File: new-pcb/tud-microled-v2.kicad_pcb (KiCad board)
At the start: 2 copper layers, 95 x 95 mm, 187 parts

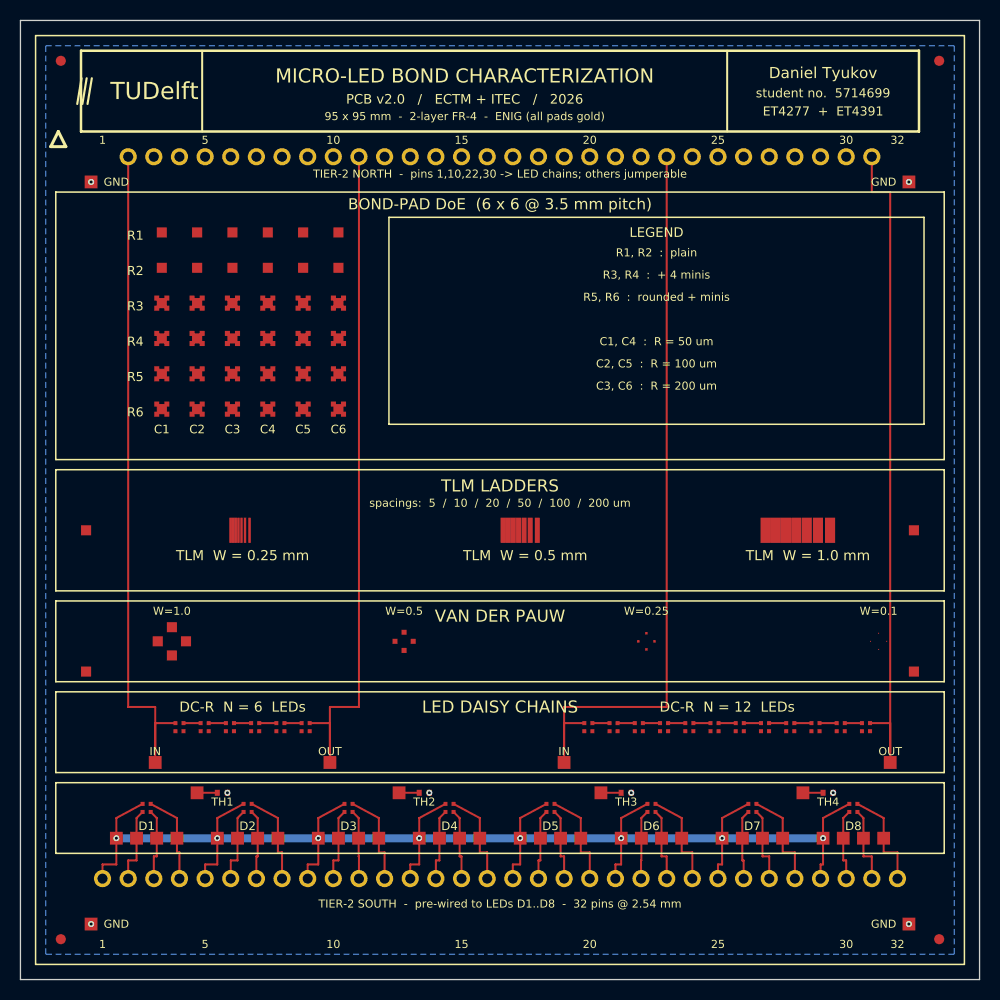
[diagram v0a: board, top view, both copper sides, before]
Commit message: Refactor code structure for improved readability and maintainability
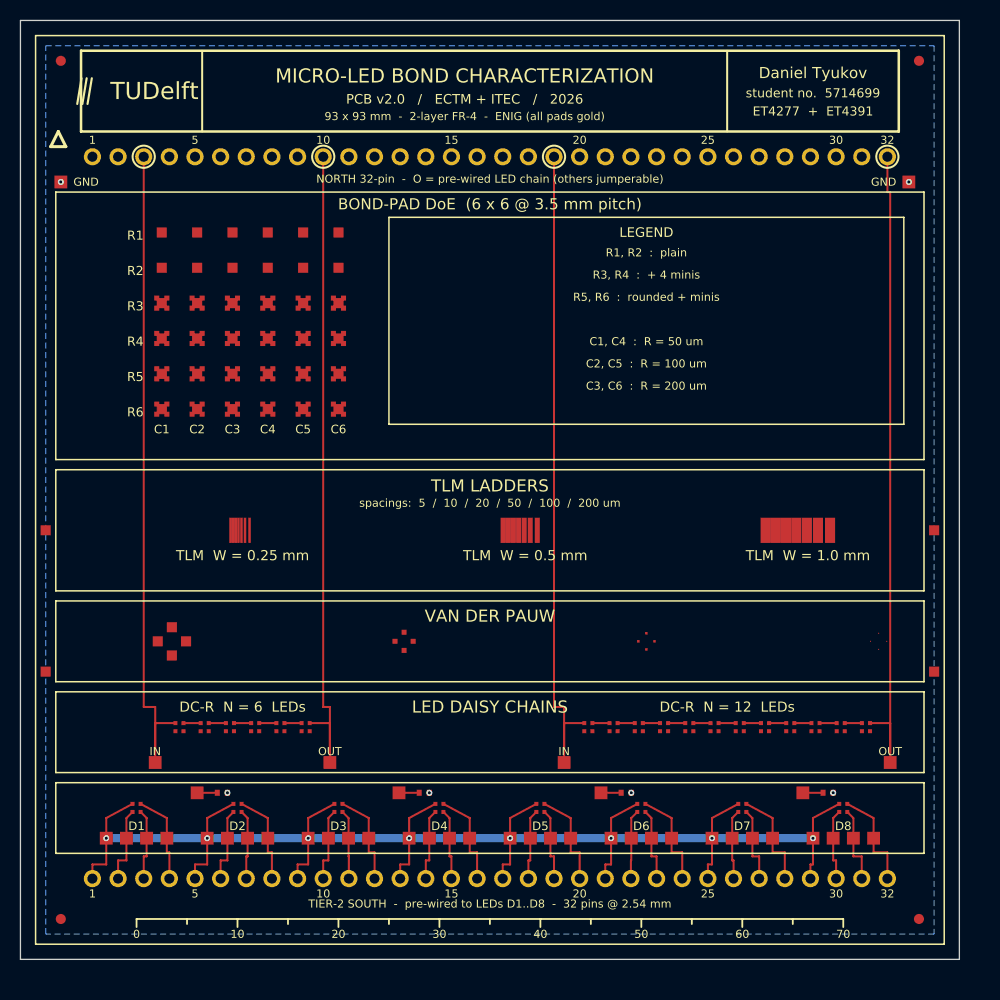
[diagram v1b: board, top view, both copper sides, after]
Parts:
- removed PP_GND3: PP_GND3, Probe_1.27mm
- removed PP_GND4: PP_GND4, Probe_1.27mm
- added H_N_31: H_N_31, Header_2.54mm, F.Cu at (83.3, 13.5)
- added H_N_32: H_N_32, Header_2.54mm, F.Cu at (85.9, 13.5)
- moved TC1 4.00 mm to (2.50, 50.5)
- moved TC2 4.00 mm to (2.50, 64.5)
- moved H_N_16 3.54 mm to (45.2, 13.5)
- moved H_N_22 3.54 mm to (60.5, 13.5)
- moved H_N_24 3.54 mm to (65.5, 13.5)
- moved H_N_26 3.54 mm to (70.6, 13.5)
- moved H_N_28 3.54 mm to (75.7, 13.5)
- moved H_N_29 3.54 mm to (78.2, 13.5)
- moved H_N_10 3.54 mm to (30.0, 13.5)
- moved H_N_6 3.54 mm to (19.8, 13.5)
- moved H_N_2 3.54 mm to (9.67, 13.5)
- moved H_N_1 3.54 mm to (7.13, 13.5)
- moved H_N_11 3.54 mm to (32.5, 13.5)
- moved H_N_12 3.54 mm to (35.1, 13.5)
- moved H_N_13 3.54 mm to (37.6, 13.5)
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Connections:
- H_N_1 pad 1: DCL6_IN -> (no net)
- H_N_19 pad 1: (no net) -> DCL12_IN
- H_N_22 pad 1: DCL12_IN -> (no net)
- H_N_3 pad 1: (no net) -> DCL6_IN
- H_N_30 pad 1: DCL12_OUT -> (no net)
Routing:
- net DCL12_IN: track 75.1 -> 65.9 mm
- net DCL6_OUT: track 67.8 -> 65.6 mm
- net DCL6_IN: track 67.6 -> 66.0 mm
- net DCL12_OUT: track 66.7 -> 65.2 mm
- net GND: vias 8 -> 6
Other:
- board size 95 x 95 mm -> 93 x 93 mm
- board text added: "0"
- board text added: "40"
- board text added: "50"
- board text added: "60"
- board text added: "70"
- board text added: "93 x 93 mm - 2-layer FR-4 - ENIG (all pads gold)"
- board text added: "NORTH 32-pin - O = pre-wired LED chain (others jumperable)"
- board text removed: "95 x 95 mm - 2-layer FR-4 - ENIG (all pads gold)"
- board text removed: "TH1"
- board text removed: "TH2"
- board text removed: "TH3"
- board text removed: "TH4"
- board text removed: "TIER-2 NORTH - pins 1,10,22,30 -> LED chains; others jumperable"
- board text removed: "W=0.1"
- board text removed: "W=0.25"
- board text removed: "W=0.5"
- board text removed: "W=1.0"
